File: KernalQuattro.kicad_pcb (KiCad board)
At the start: 2 copper layers, 18.3 x 31 mm, 16 parts, among them CN1 2364, J1 Conn, SW1 DIP Switch, U1 28C256

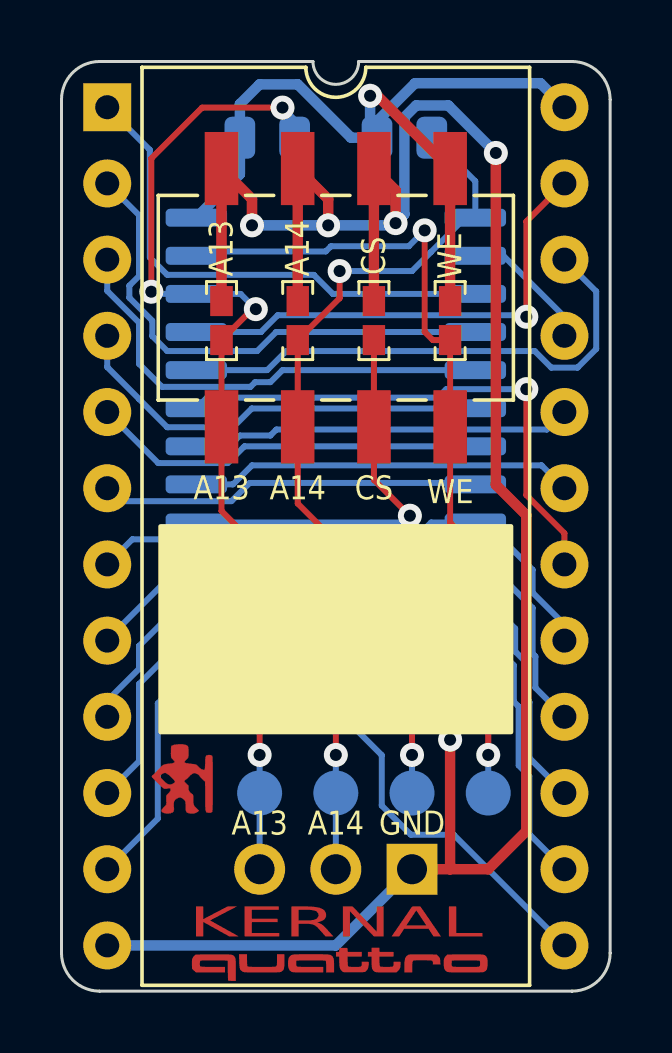
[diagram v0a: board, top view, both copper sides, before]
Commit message: Work in progress.
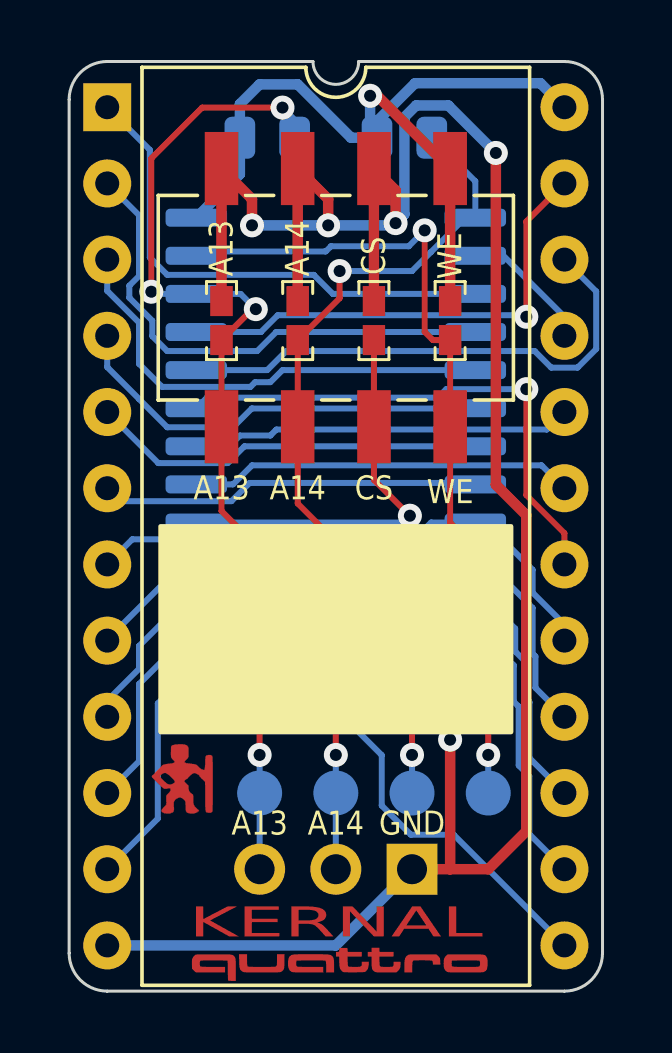
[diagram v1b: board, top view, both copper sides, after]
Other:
- board size 18.3 x 31 mm -> 17.8 x 31 mm
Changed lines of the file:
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@@
     ) (layer "F.SilkS") (width 0.15) (fill solid))
   (gr_arc (start 119.126 60.96) (mid 118.364 61.722) (end 117.602 60.96) (layer "Edge.Cuts") (width 0.1))
-  (gr_arc (start 109.22 62.23) (mid 109.591974 61.331974) (end 110.49 60.96) (layer "Edge.Cuts") (width 0.1))
-  (gr_arc (start 127.508 90.678) (mid 127.136026 91.576026) (end 126.238 91.948) (layer "Edge.Cuts") (width 0.1))
-  (gr_arc (start 110.49 91.948) (mid 109.591974 91.576026) (end 109.22 90.678) (layer "Edge.Cuts") (width 0.1))
-  (gr_line (start 127.508 62.23) (end 127.508 90.678) (layer "Edge.Cuts") (width 0.1))
-  (gr_arc (start 126.238 60.96) (mid 127.136026 61.331974) (end 127.508 62.23) (layer "Edge.Cuts") (width 0.1))
-  (gr_line (start 126.238 60.96) (end 119.126 60.96) (layer "Edge.Cuts") (width 0.1))
-  (gr_line (start 126.238 91.948) (end 110.49 91.948) (layer "Edge.Cuts") (width 0.1))
-  (gr_line (start 110.49 60.96) (end 117.602 60.96) (layer "Edge.Cuts") (width 0.1))
-  (gr_line (start 109.22 90.678) (end 109.22 62.23) (layer "Edge.Cuts") (width 0.1))
+  (gr_arc (start 109.474 62.23) (mid 109.845974 61.331974) (end 110.744 60.96) (layer "Edge.Cuts") (width 0.1))
+  (gr_arc (start 127.254 90.678) (mid 126.882026 91.576026) (end 125.984 91.948) (layer "Edge.Cuts") (width 0.1))
+  (gr_arc (start 110.744 91.948) (mid 109.845974 91.576026) (end 109.474 90.678) (layer "Edge.Cuts") (width 0.1))
+  (gr_line (start 127.254 62.23) (end 127.254 90.678) (layer "Edge.Cuts") (width 0.1))
+  (gr_arc (start 125.984 60.96) (mid 126.882026 61.331974) (end 127.254 62.23) (layer "Edge.Cuts") (width 0.1))
+  (gr_line (start 125.984 60.96) (end 119.126 60.96) (layer "Edge.Cuts") (width 0.1))
+  (gr_line (start 125.984 91.948) (end 110.744 91.948) (layer "Edge.Cuts") (width 0.1))
+  (gr_line (start 110.744 60.96) (end 117.602 60.96) (layer "Edge.Cuts") (width 0.1))
+  (gr_line (start 109.474 90.678) (end 109.474 62.23) (layer "Edge.Cuts") (width 0.1))
   (gr_text "KERNAL" (at 118.364 89.662) (layer "F.Cu")
     (effects (font (size 1 1.8) (thickness 0.25)))
@@
   (segment (start 125.984 69.469) (end 123.952 67.437) (width 0.2) (layer "B.Cu") (net 20))
   (segment (start 125.984 70.104) (end 125.984 69.469) (width 0.2) (layer "B.Cu") (net 20))
+  (segment (start 116.712148 70.612) (end 124.993624 70.612) (width 0.2) (layer "B.Cu") (net 21))
   (segment (start 124.993624 70.612) (end 125.545135 71.163511) (width 0.2) (layer "B.Cu") (net 21))
-  (segment (start 116.712148 70.612) (end 124.993624 70.612) (width 0.2) (layer "B.Cu") (net 21))
   (segment (start 127.043511 68.623511) (end 125.984 67.564) (width 0.2) (layer "B.Cu") (net 21))
   (segment (start 113.714 71.247) (end 116.077148 71.247) (width 0.2) (layer "B.Cu") (net 21))
